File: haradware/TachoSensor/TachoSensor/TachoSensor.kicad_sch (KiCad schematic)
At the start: 1 part, among them J101 OUT

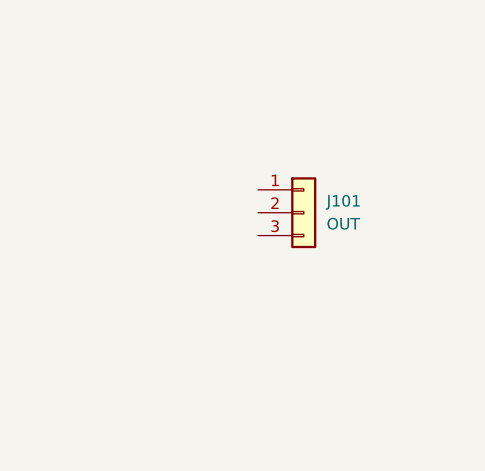
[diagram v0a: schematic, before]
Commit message: センサーの基板作成 確認後発注可能
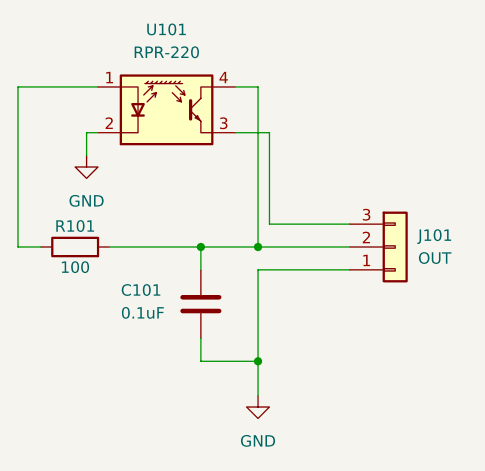
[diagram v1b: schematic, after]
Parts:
- added C101: 0.1uF, Capacitor_THT:C_Axial_L3.8mm_D2.6mm_P7.50mm_Horizontal, symbol Device:C
- added R101: 100, Resistor_THT:R_Axial_DIN0207_L6.3mm_D2.5mm_P10.16mm_Horizontal, symbol Device:R
- added U101: RPR-220, OptoDevice:Everlight_ITR8307F43, symbol Sensor_Proximity:BPR-105F
- J101: footprint (none) -> Connector_JST:JST_XH_S3B-XH-A-1_1x03_P2.50mm_Horizontal
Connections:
- net GND: now reaches J101.1 (Pin_3)
- net GND: now also C101.2, U101.2 (K)
- net at J101.2 (Pin_2): now also C101.1, R101.2, U101.4 (4C)
- net at J101.3 (Pin_1): now also U101.3 (E)
- new net: R101.1, U101.1 (A)
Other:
- moved on the sheet: J101
